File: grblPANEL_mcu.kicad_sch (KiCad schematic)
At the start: 28 parts, among them J201 2x5x1.27mm, J202 USB_C_Receptacle_USB2.0, SW201 SW_Push, SW202 SW_Push, U201 STM32G0B1CxTxN, U202 USBLC6-2SC6, Y201 8MHz

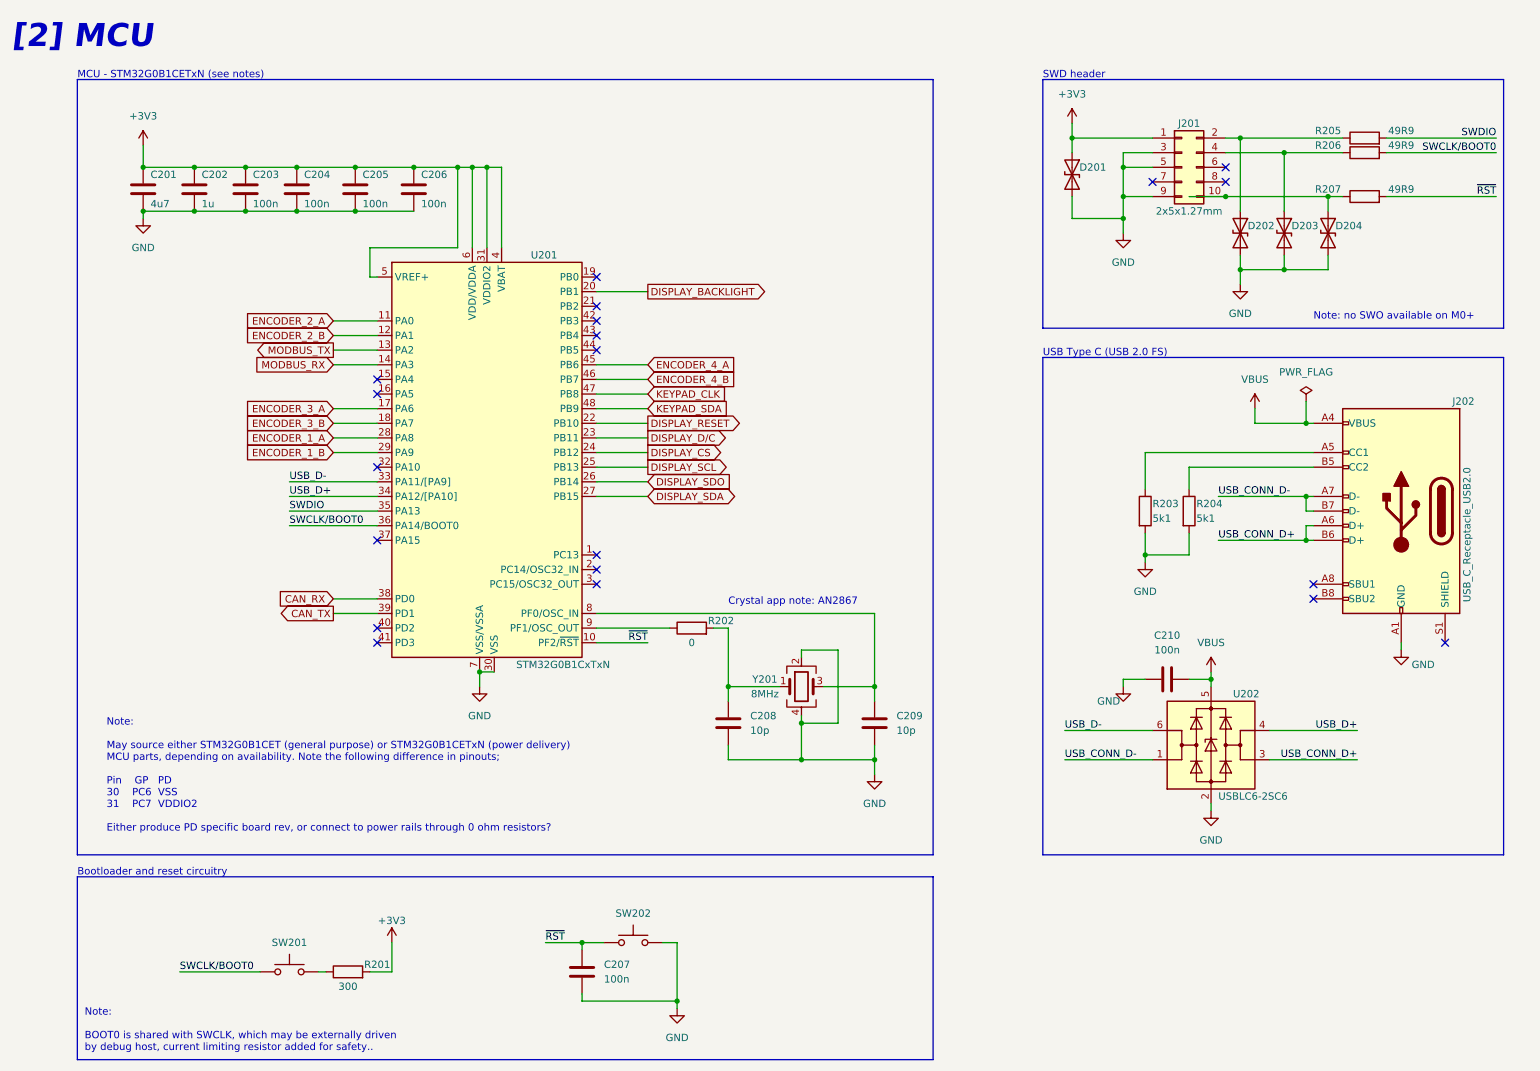
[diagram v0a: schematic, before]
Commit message: Refresh
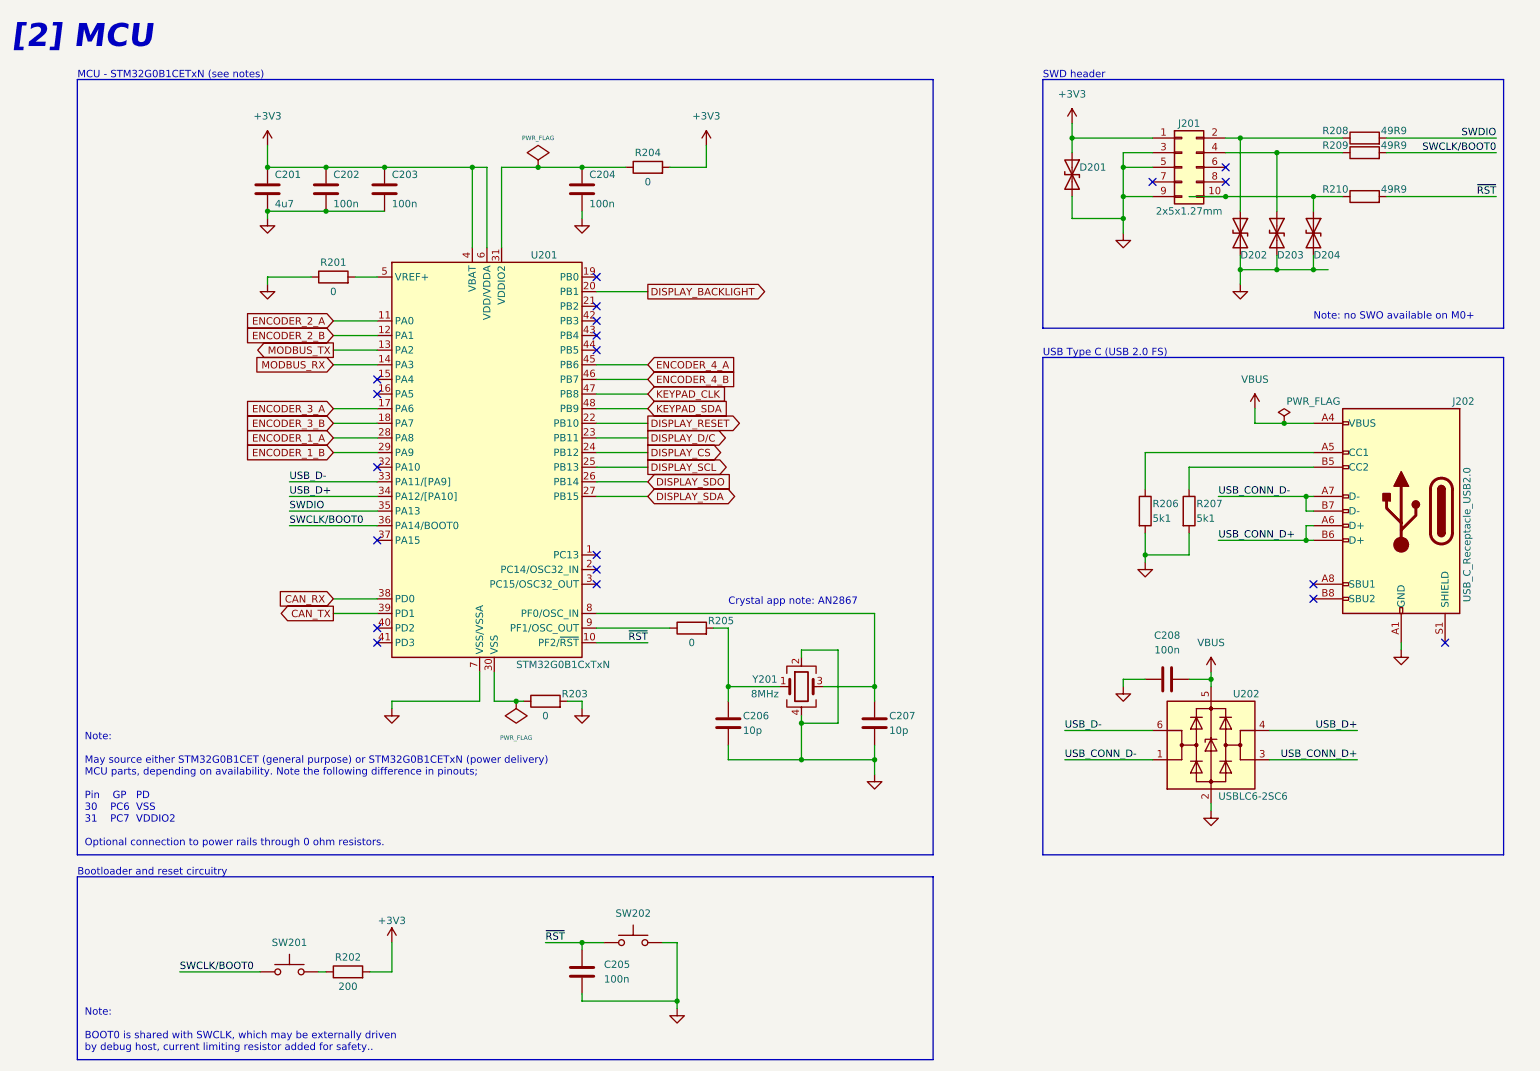
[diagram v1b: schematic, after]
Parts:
- removed C202: 1u, symbol Device:C
- removed C203, C206: 100n, symbol Device:C
- added C204: 100n, Capacitor_SMD:C_0603_1608Metric, symbol Device:C
- added R201, R203, R204: 0, Resistor_SMD:R_0603_1608Metric, symbol Device:R
- C201: footprint (none) -> Capacitor_SMD:C_0805_2012Metric
- C202: renamed from C204; footprint (none) -> Capacitor_SMD:C_0603_1608Metric
- C203: renamed from C205; footprint (none) -> Capacitor_SMD:C_0603_1608Metric
- C205: renamed from C207; footprint (none) -> Capacitor_SMD:C_0603_1608Metric
- C206: renamed from C208; footprint (none) -> Capacitor_SMD:C_0603_1608Metric
- C207: renamed from C209; footprint (none) -> Capacitor_SMD:C_0603_1608Metric
- C208: renamed from C210; footprint (none) -> Capacitor_SMD:C_0603_1608Metric
- D201, D202, D203, D204: footprint (none) -> Diode_SMD:D_SOD-323
- J201: footprint (none) -> dresco:FTSH-105-01-L-DV-K
- J202: footprint (none) -> Connector_USB:USB_C_Receptacle_HRO_TYPE-C-31-M-12
- R202: renamed from R201; value 300 -> 200; footprint (none) -> Resistor_SMD:R_0603_1608Metric
- R205: renamed from R202; footprint (none) -> Resistor_SMD:R_0603_1608Metric
- R206: renamed from R203; footprint (none) -> Resistor_SMD:R_0603_1608Metric
- R207: renamed from R204; footprint (none) -> Resistor_SMD:R_0603_1608Metric
- R208: renamed from R205; footprint (none) -> Resistor_SMD:R_0603_1608Metric
- R209: renamed from R206; footprint (none) -> Resistor_SMD:R_0603_1608Metric
- R210: renamed from R207; footprint (none) -> Resistor_SMD:R_0603_1608Metric
- SW201, SW202: footprint (none) -> Connector_Pin:Pin_D1.0mm_L10.0mm_LooseFit
- Y201: footprint (none) -> Crystal:Crystal_SMD_3225-4Pin_3.2x2.5mm
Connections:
- net +3V3: now also R204.2; no longer U201.31 (VDDIO2), U201.5 (VREF+)
- net GND: now also C204.2, R201.1, R203.2; no longer U201.30 (VSS)
- new net: C204.1, R204.1, U201.31 (VDDIO2)
- new net: R203.1, U201.30 (VSS)
- new net: R201.2, U201.5 (VREF+)
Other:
- note added: "Note: May source either STM32G0B1CET (general purpose) or STM32G0B1CETxN (power delivery) MCU parts, depending on availability. Note the following difference in pinouts; Pin GP PD 30 PC6 VSS 31 PC7 VDDIO2 Optional connection to power rails through 0 ohm resistors."
- note removed: "Note: May source either STM32G0B1CET (general purpose) or STM32G0B1CETxN (power delivery) MCU parts, depending on availability. Note the following difference in pinouts; Pin GP PD 30 PC6 VSS 31 PC7 VDDIO2 Either produce PD specific board rev, or connect to power rails through 0 ohm resistors?"
- moved on the sheet: C201, C202, C203, D203, D204
